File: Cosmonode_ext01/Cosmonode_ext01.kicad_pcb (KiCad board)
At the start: 2 copper layers, 12.7 x 10.2 mm, 4 parts, among them J1 CONN_01X04, J2 CONN_01X01, J3 GS3, U1 SI7020-A20-YM0R

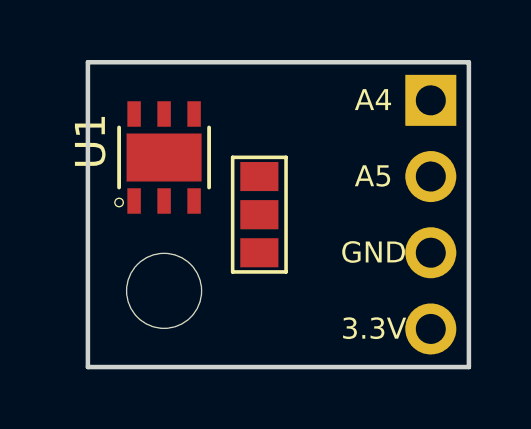
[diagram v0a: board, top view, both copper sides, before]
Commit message: start v0.8
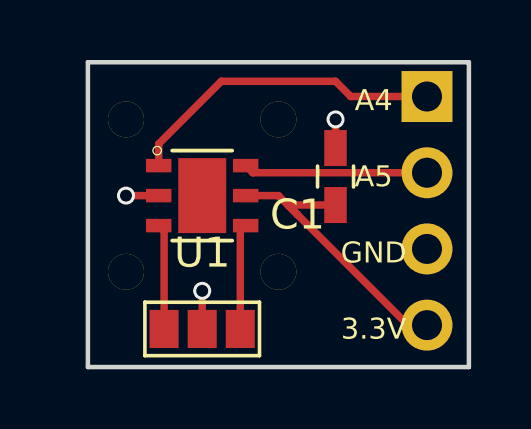
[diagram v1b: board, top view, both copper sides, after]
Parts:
- added C1: 100nF, Capacitors_SMD:C_0603_HandSoldering, F.Cu at (170.2, 104.8)
- added J4: CONN_01X01, Wire_Pads:SolderWirePad_single_1-2mmDrill, F.Cu at (168.3, 108.0)
- added J5: CONN_01X01, Wire_Pads:SolderWirePad_single_1-2mmDrill, F.Cu at (163.2, 102.9)
- added J6: CONN_01X01, Wire_Pads:SolderWirePad_single_1-2mmDrill, F.Cu at (168.3, 102.9)
- J2: footprint Mounting_Holes:MountingHole_2.5mm -> Wire_Pads:SolderWirePad_single_1-2mmDrill
- moved J3 4.26 mm to (165.7, 109.9), turned to 270 degrees
- moved U1 1.80 mm to (165.7, 105.4), turned to 0 degrees
- moved J2 1.42 mm to (163.2, 108.0)
- moved J1 0.18 mm to (173.2, 102.1)
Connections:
- U1 pad 7: GND -> Net-(U1-Pad7)
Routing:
- net A4: track 0.00 -> 10.7 mm
- net +3V3: track 0.00 -> 9.87 mm
- net A5: track 0.00 -> 6.14 mm
- net Net-(J3-Pad3): track 0.00 -> 3.52 mm
- net Net-(J3-Pad1): track 0.00 -> 3.52 mm
- net GND: track 0.00 -> 3.32 mm, vias 0 -> 3
- added copper zone on B.Cu, net GND
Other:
- board text added: "A commander en 1.2 mm d'épaisseur"
